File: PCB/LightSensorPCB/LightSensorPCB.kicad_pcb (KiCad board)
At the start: 2 copper layers, 20 x 23 mm, 15 parts, among them J1 POWER/I2C, U1 LTR-329ALS-01, U2 LSM6DSMTR, U3 VL53L3CXV0DH/1

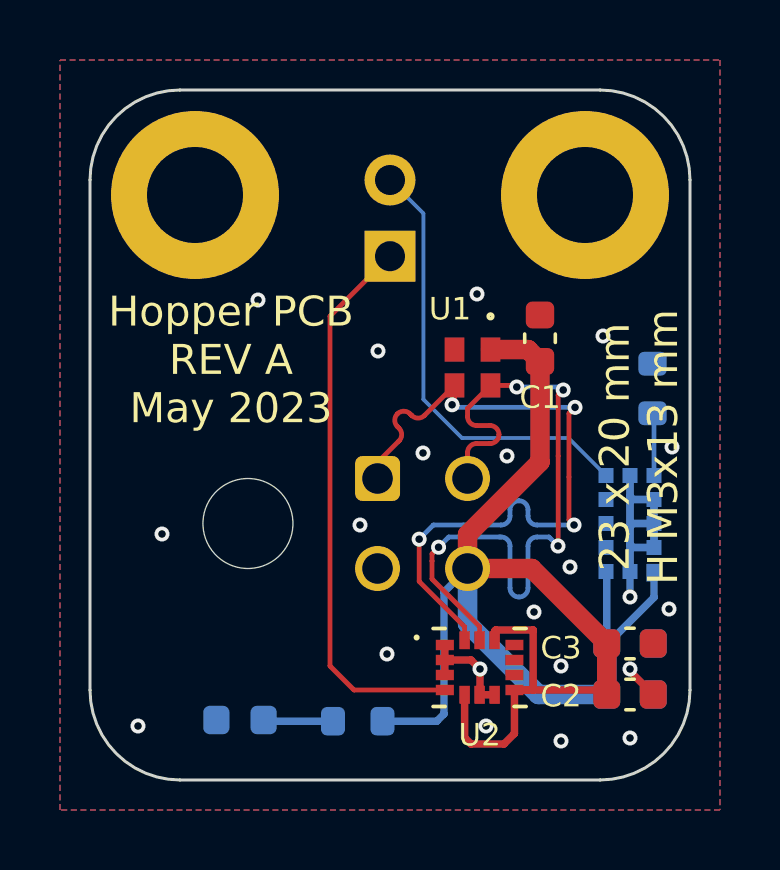
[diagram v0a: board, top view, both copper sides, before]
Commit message: 3x PCB ordered
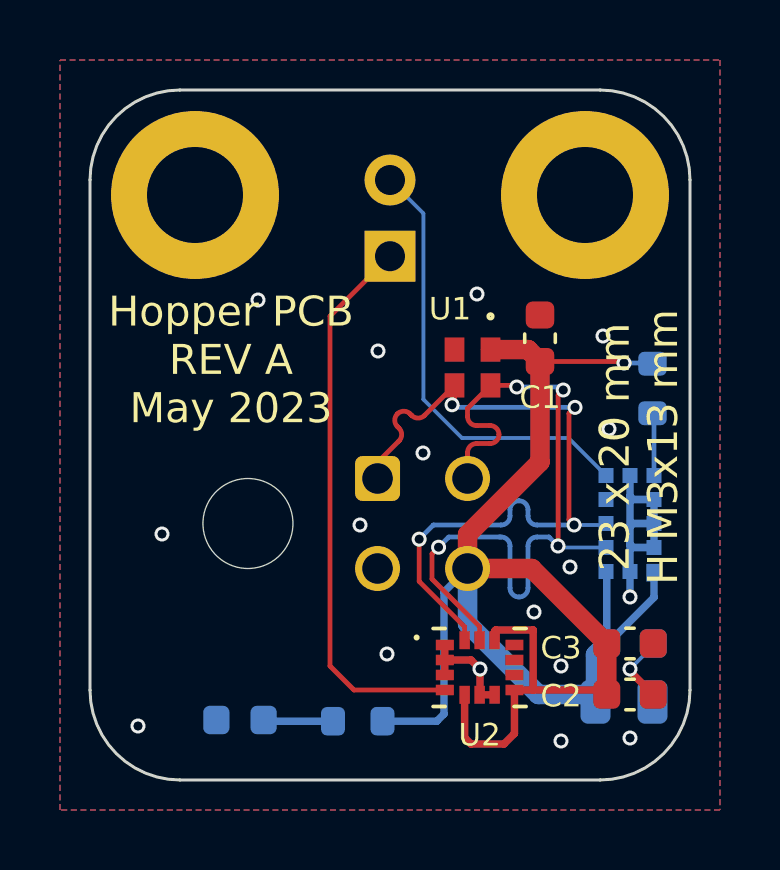
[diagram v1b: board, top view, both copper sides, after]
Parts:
- C4: value 4.7 uF 6.3V X5R 0603 -> 4.7 uF 25V X5R 0805; footprint Capacitor_SMD:C_0603_1608Metric -> Capacitor_SMD:C_0805_2012Metric
- moved C4 0.32 mm to (117.8, 120.4)
- turned R4 to 90 degrees
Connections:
- R4 pad 1: GND -> Net-(U3-Pad5)
- R4 pad 2: Net-(U3-Pad5) -> +3.3V
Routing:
- net +3.3V: track 51.5 -> 54.2 mm, vias 0 -> 1
- net /SCL: track 24.2 -> 25.9 mm
- net GND: track 13.0 -> 14.1 mm, vias 20 -> 18
- net (no net): vias 1 -> 0
